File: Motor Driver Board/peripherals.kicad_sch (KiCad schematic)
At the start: 1 part, among them U2 SN65HVD230

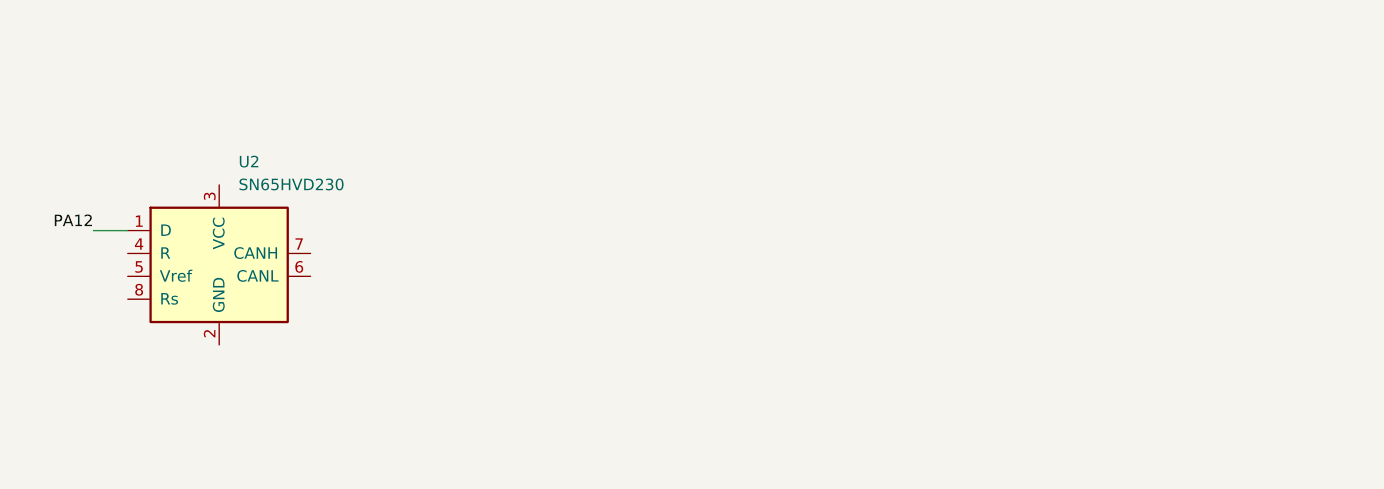
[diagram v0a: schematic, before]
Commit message: updated pcb
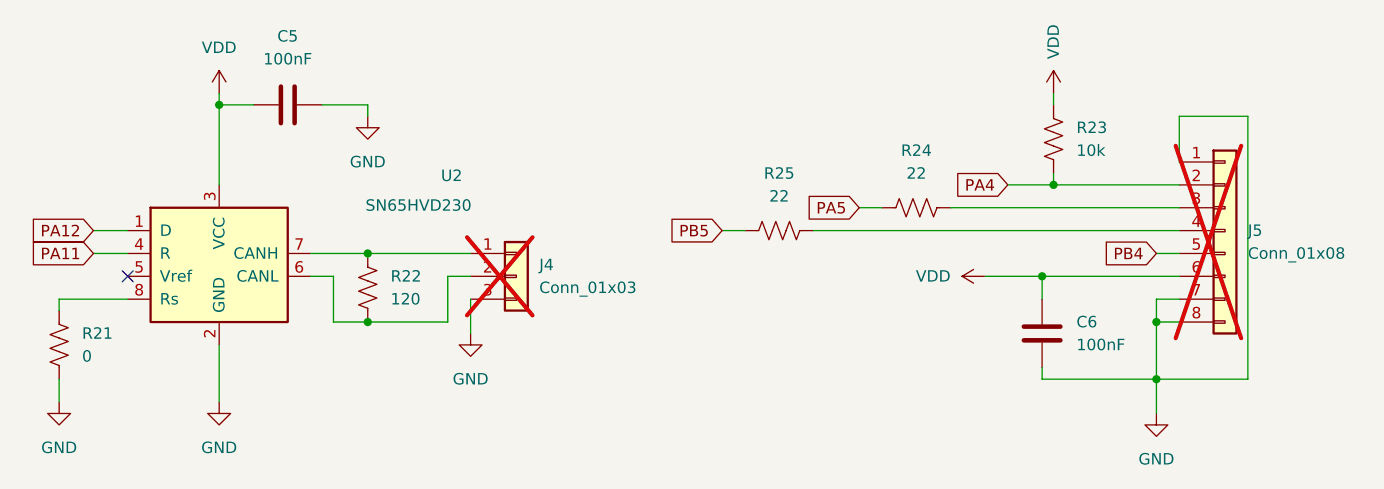
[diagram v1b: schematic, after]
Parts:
- added C5, C6: 100nF, Capacitor_SMD:C_0402_1005Metric, symbol Device:C
- added J4: Conn_01x03, Connector_PinHeader_2.54mm:PinHeader_1x03_P2.54mm_Vertical, symbol Connector_Generic:Conn_01x03
- added J5: Conn_01x08, Connector_PinHeader_2.54mm:PinHeader_1x08_P2.54mm_Horizontal, symbol Connector_Generic:Conn_01x08
- added R21: 0, Resistor_SMD:R_0805_2012Metric, symbol Device:R_US
- added R22: 120, Resistor_SMD:R_0805_2012Metric, symbol Device:R_US
- added R23: 10k, Resistor_SMD:R_0805_2012Metric, symbol Device:R_US
- added R24, R25: 22, Resistor_SMD:R_0805_2012Metric, symbol Device:R_US
- U2: LCSC (none) -> C12084
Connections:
- net GND: now reaches U2.2 (GND)
- net GND: now also C5.2, C6.2, J4.3 (Pin_3), J5.1 (Pin_1), J5.7 (Pin_7), J5.8 (Pin_8), R21.2
- net VDD: now reaches U2.3 (VCC)
- net VDD: now also C5.1, C6.1, J5.6 (Pin_6), R23.1
- net PA11: now reaches U2.4 (R)
- net at U2.6 (CANL): now also J4.2 (Pin_2), R22.2
- net at U2.7 (CANH): now also J4.1 (Pin_1), R22.1
- net at U2.8 (Rs): now also R21.1
- new net: J5.3 (Pin_3), R24.2
- new net: J5.4 (Pin_4), R25.2
- new net PA4: J5.2 (Pin_2), R23.2
- new net PA5: R24.1
- new net PB4: J5.5 (Pin_5)
- new net PB5: R25.1
- no-connect marks 0 -> 1
